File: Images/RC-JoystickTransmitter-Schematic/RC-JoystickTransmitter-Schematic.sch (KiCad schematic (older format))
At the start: 9 parts

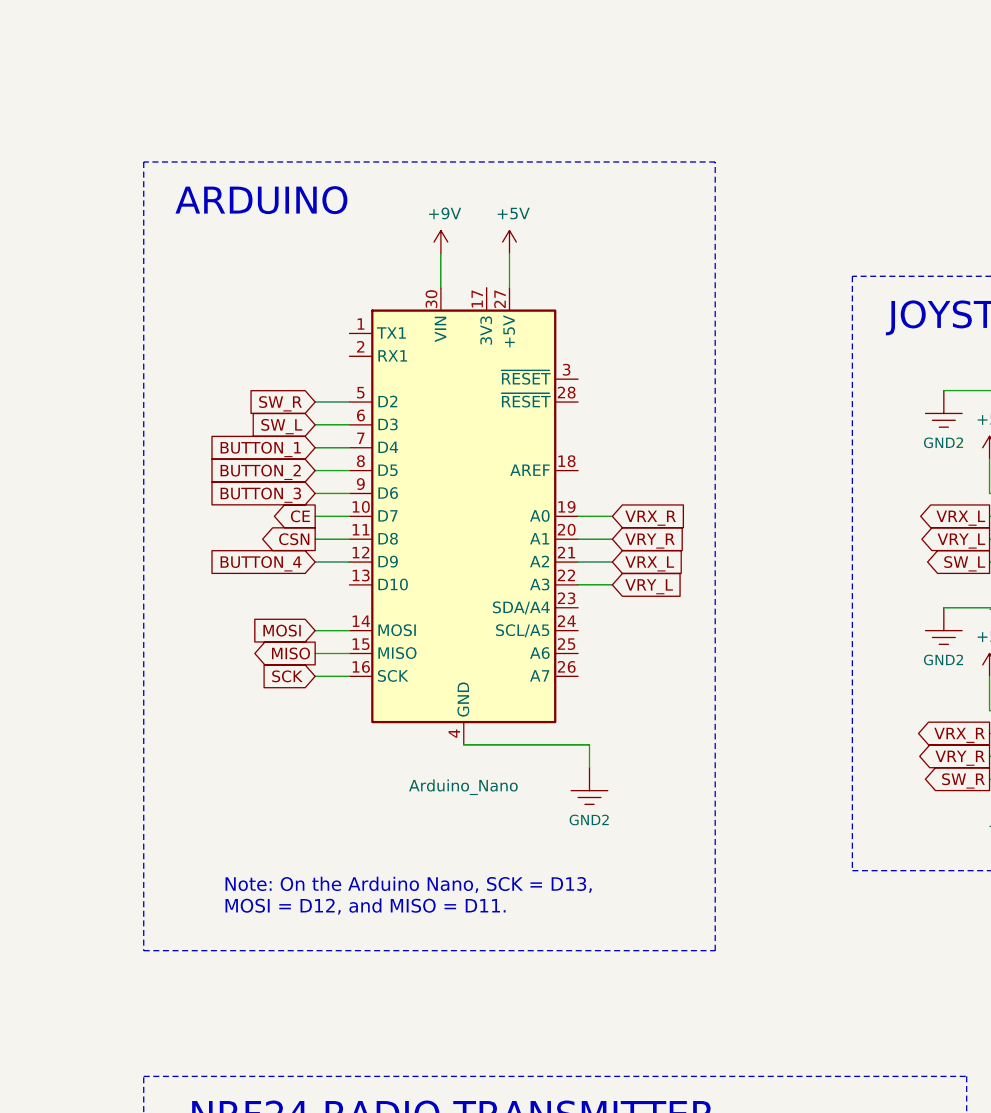
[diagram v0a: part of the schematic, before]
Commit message: Update schematic
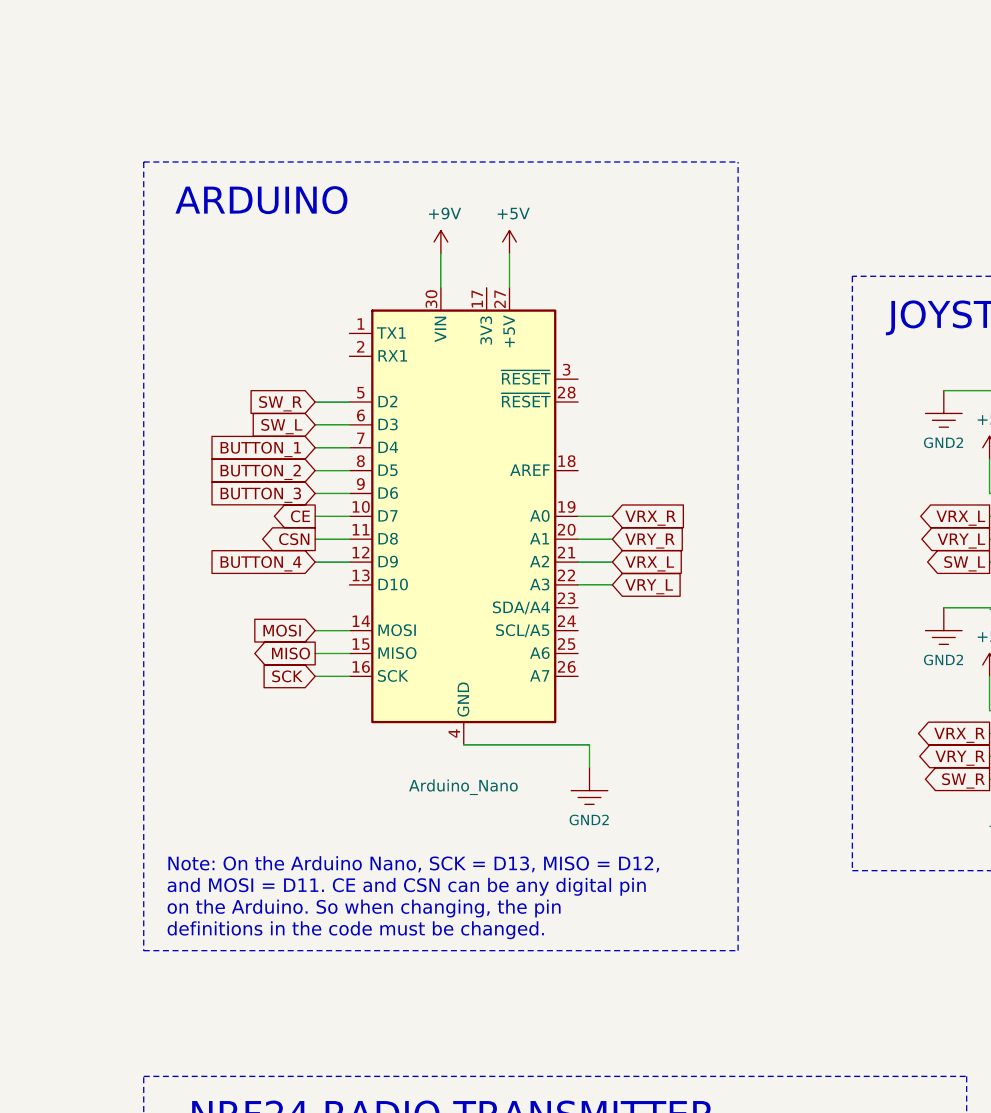
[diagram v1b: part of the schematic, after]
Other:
- note added: "Note: On the Arduino Nano, SCK = D13, MISO = D12, \nand MOSI = D11. CE and CSN can be any digital pin\non the Arduino. So when changing, the pin \ndefinitions in the code must be changed."
- note removed: "Note: On the Arduino Nano, SCK = D13, \nMOSI = D12, and MISO = D11."
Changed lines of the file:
@@
 	4500 2500 4500 5100
 Wire Notes Line
-	1400 5450 3900 5450
-Wire Notes Line
-	3900 5450 3900 2000
-Wire Notes Line
-	3900 2000 1400 2000
+	4000 5450 4000 2000
 Wire Notes Line
 	1400 2000 1400 5450
-Text Notes 1750 5300 0    59   ~ 0
-Note: On the Arduino Nano, SCK = D13, \nMOSI = D12, and MISO = D11.
+Text Notes 1500 5400 0    59   ~ 0
+Note: On the Arduino Nano, SCK = D13, MISO = D12, \nand MOSI = D11. CE and CSN can be any digital pin\non the Arduino. So when changing, the pin \ndefinitions in the code must be changed.
 $Comp
 L SparkFun-PowerSymbols:GND2 #GND?
@@
 Wire Wire Line
 	1750 6900 2650 6900
+Wire Notes Line
+	1400 2000 4000 2000
+Wire Notes Line
+	1400 5450 4000 5450
 $EndSCHEMATC
